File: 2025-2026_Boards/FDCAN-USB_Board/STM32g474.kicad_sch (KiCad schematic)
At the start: 14 parts, among them J4 Conn_01x02_Pin, J5 Conn_01x02_Pin, J6 Conn_ARM_JTAG_SWD_10, U3 STM32G474CETx

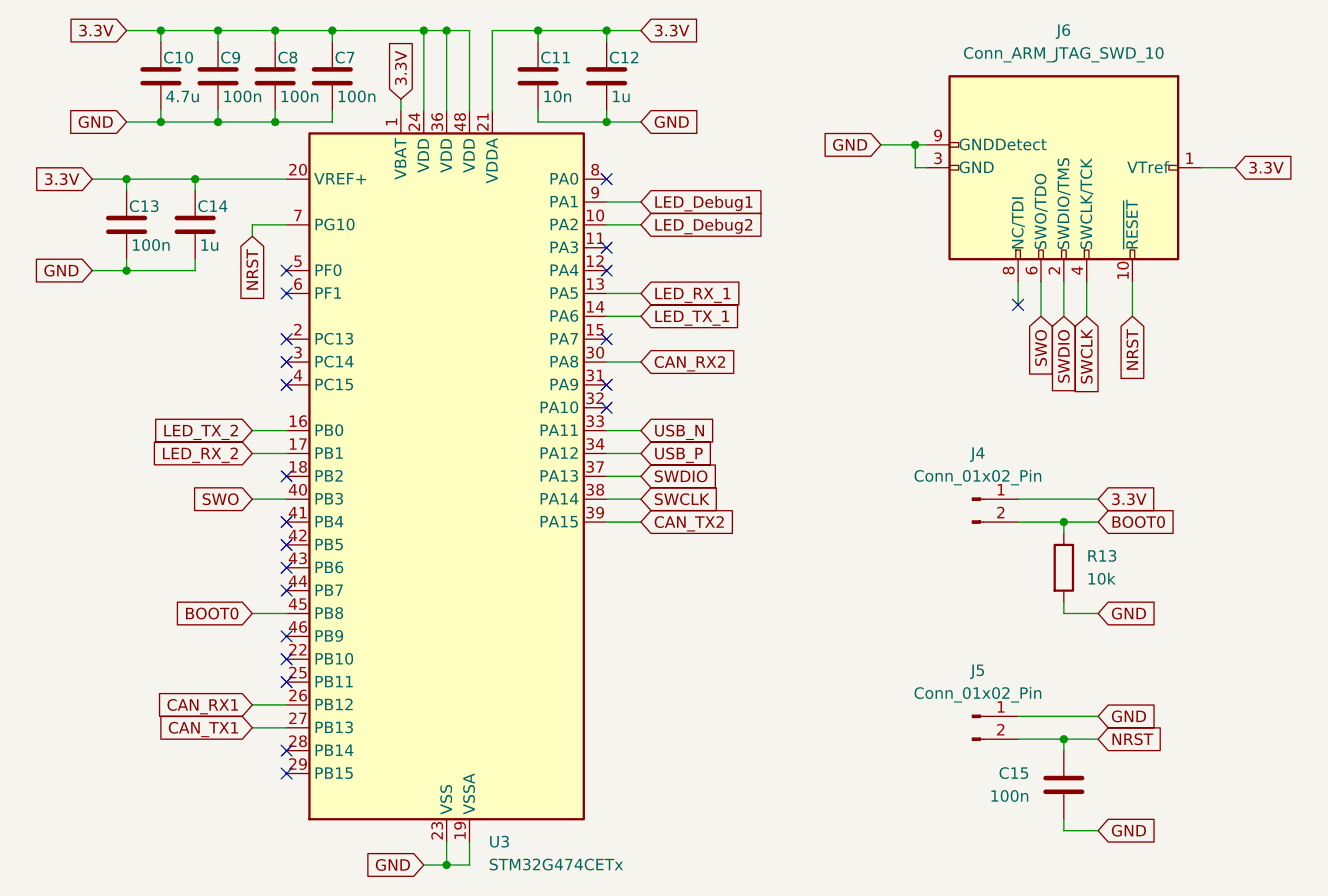
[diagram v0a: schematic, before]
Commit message: microcontroller pin update
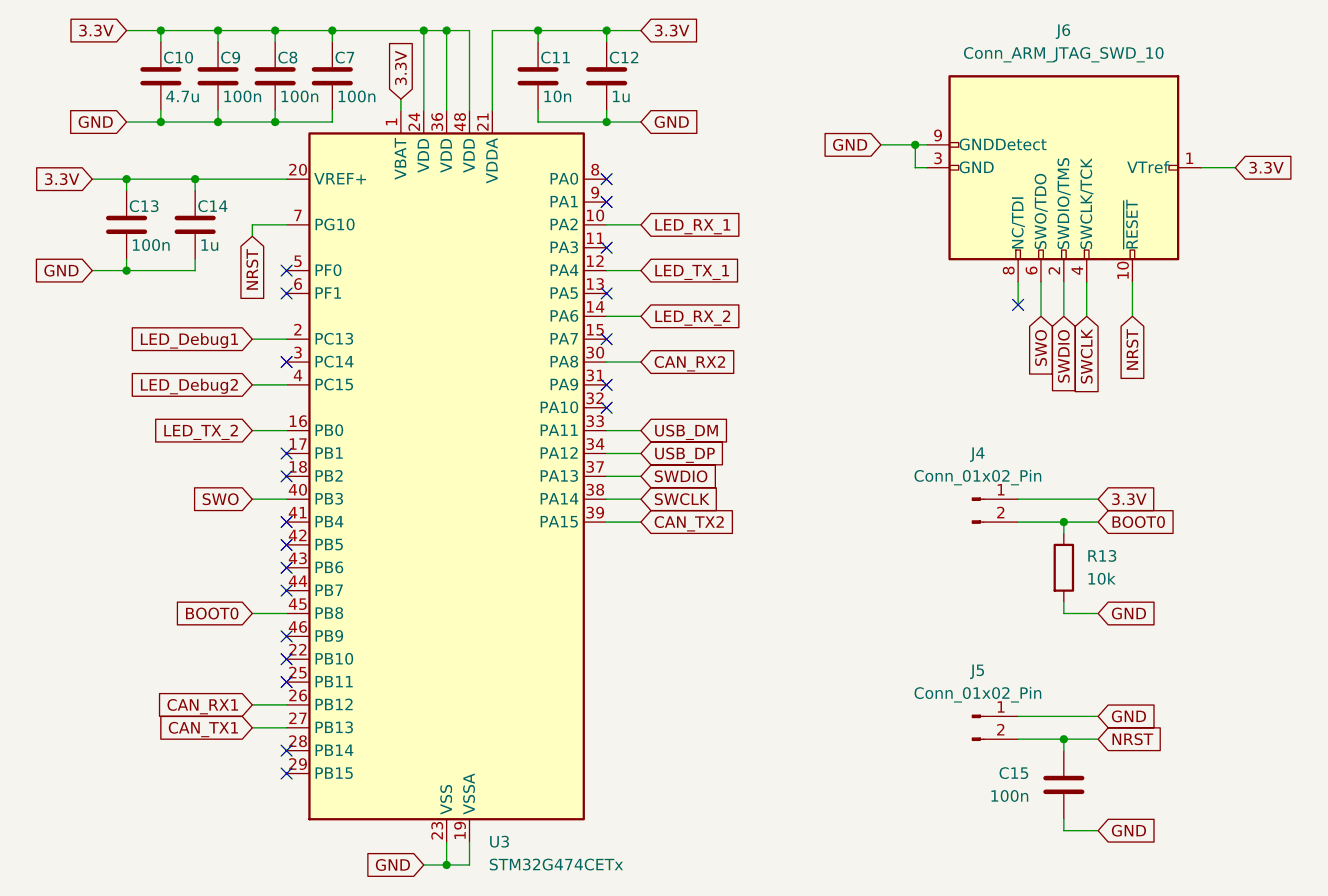
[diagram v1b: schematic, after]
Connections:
- net LED_Debug1: now also U3.2 (PC13); no longer U3.9 (PA1)
- net LED_Debug2: now also U3.4 (PC15); no longer U3.10 (PA2)
- net LED_RX_1: now also U3.10 (PA2); no longer U3.13 (PA5)
- net LED_RX_2: now also U3.14 (PA6); no longer U3.17 (PB1)
- net LED_TX_1: now also U3.12 (PA4); no longer U3.14 (PA6)
- net USB_N renamed USB_DM
- net USB_P renamed USB_DP
